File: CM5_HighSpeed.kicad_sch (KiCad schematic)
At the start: 5 parts, among them J10 690-019-298-412, U18 RT9742SNGV

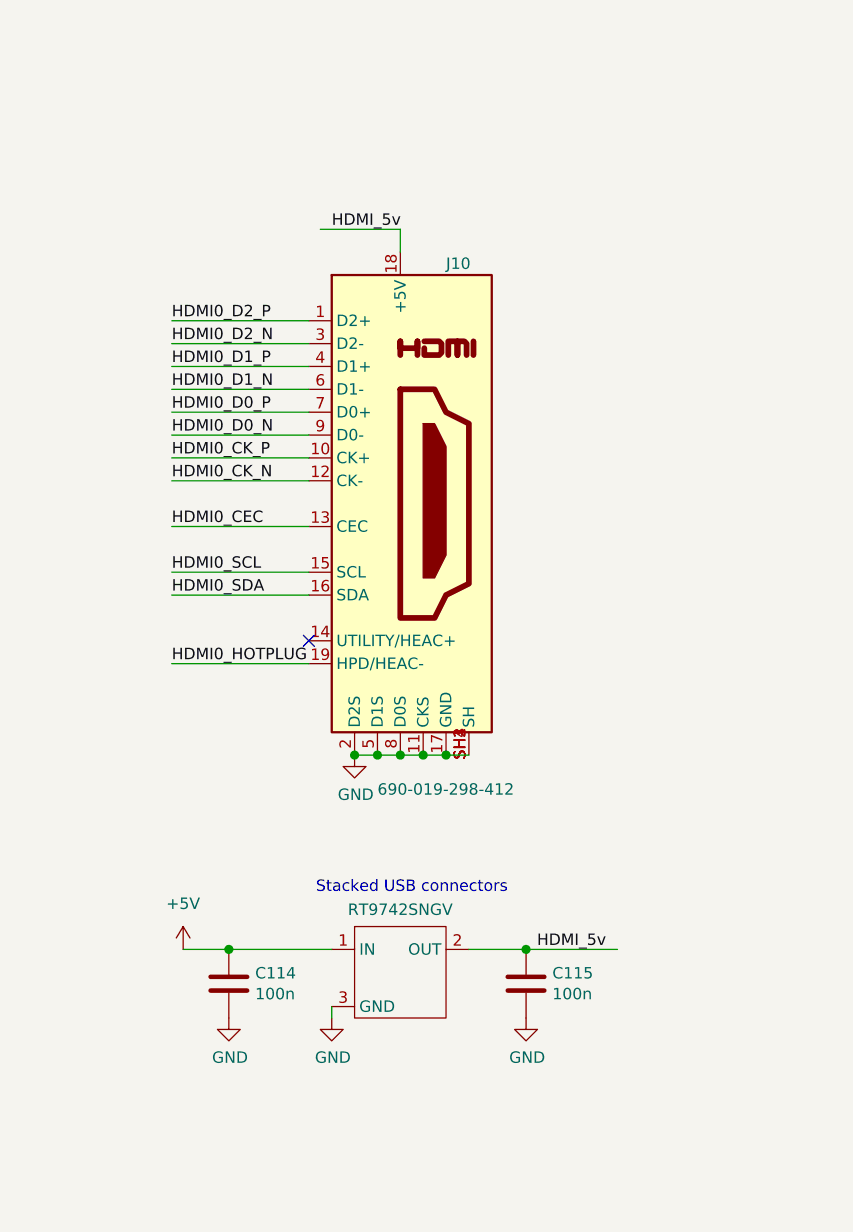
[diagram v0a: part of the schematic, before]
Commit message: change cad data
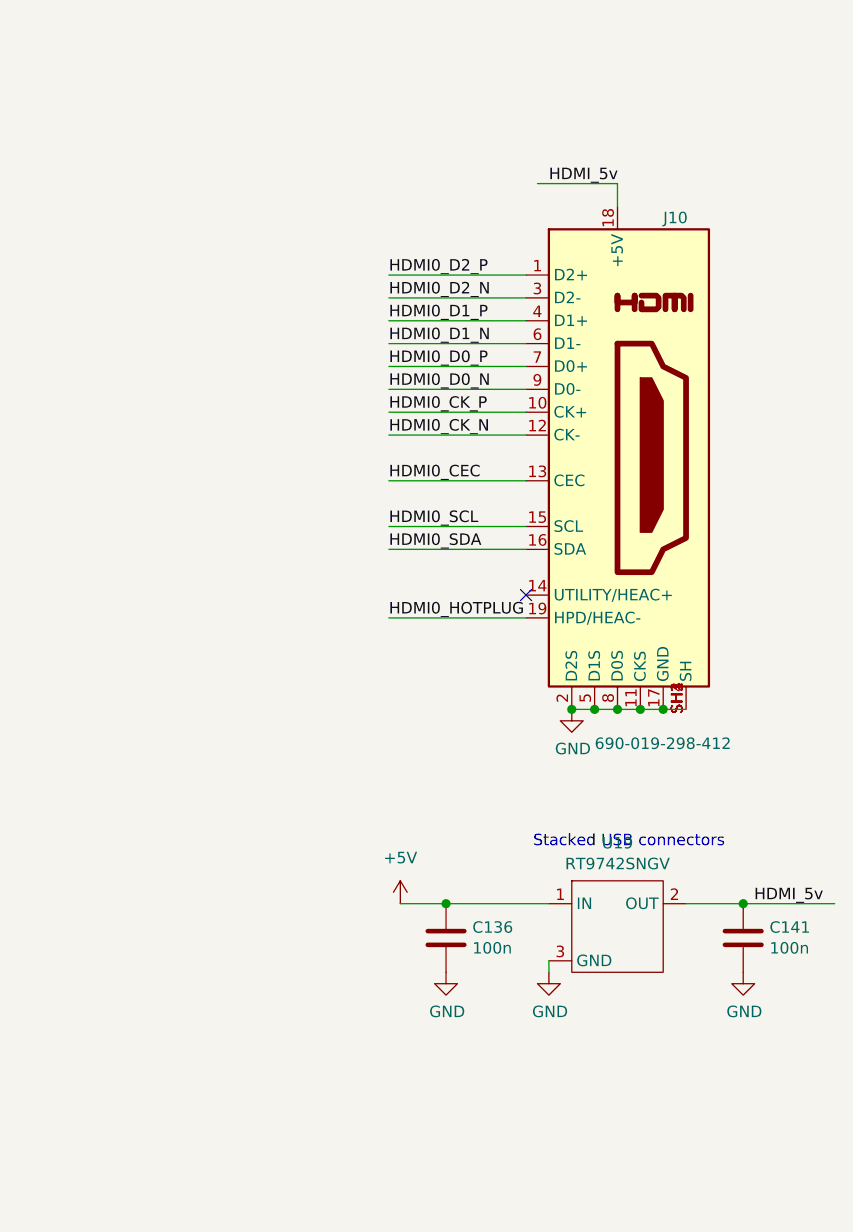
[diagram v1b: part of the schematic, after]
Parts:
- C136: renamed from C114; footprint Capacitor_SMD:C_0402_1005Metric -> Capacitor_SMD:C_0402_1005Metric_Pad0.74x0.62mm_HandSolder
- C141: renamed from C115; footprint Capacitor_SMD:C_0402_1005Metric -> Capacitor_SMD:C_0402_1005Metric_Pad0.74x0.62mm_HandSolder
- renumbered U18 to U19
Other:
- moved on the sheet: C136, C141, J10
